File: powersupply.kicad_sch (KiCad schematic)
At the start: 94 parts, among them J201 EXT PWR, U201 TPS54332, U202 TPS54332, U203 TPS54332, U204 TPS54332

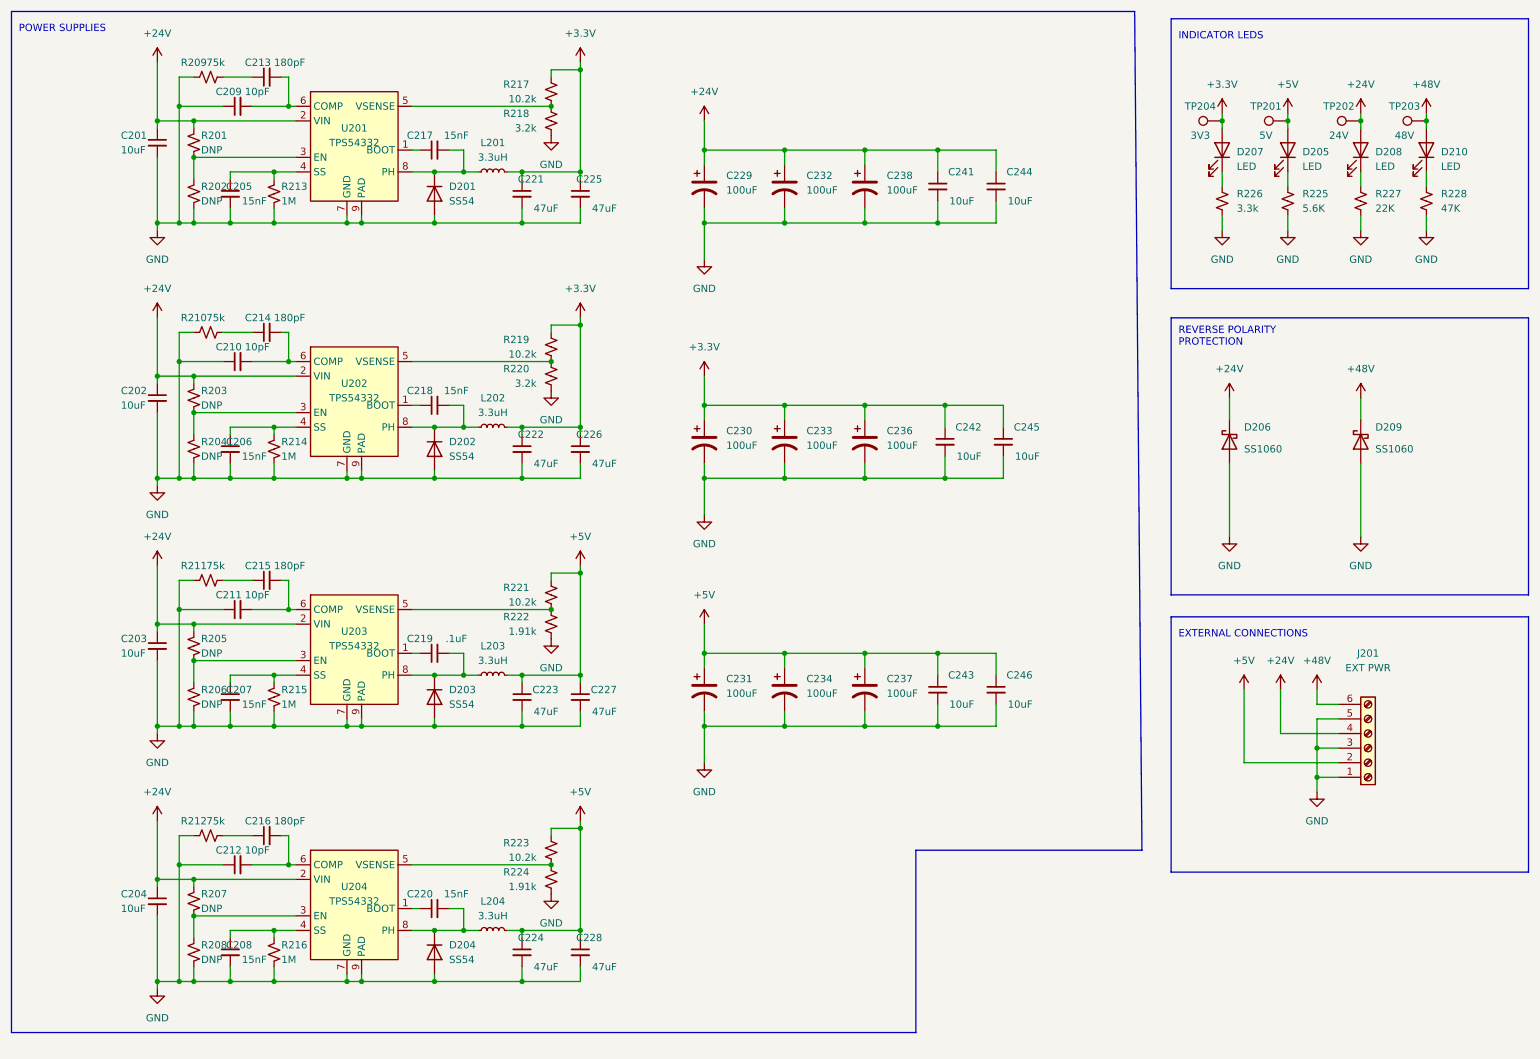
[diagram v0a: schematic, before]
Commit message: update board
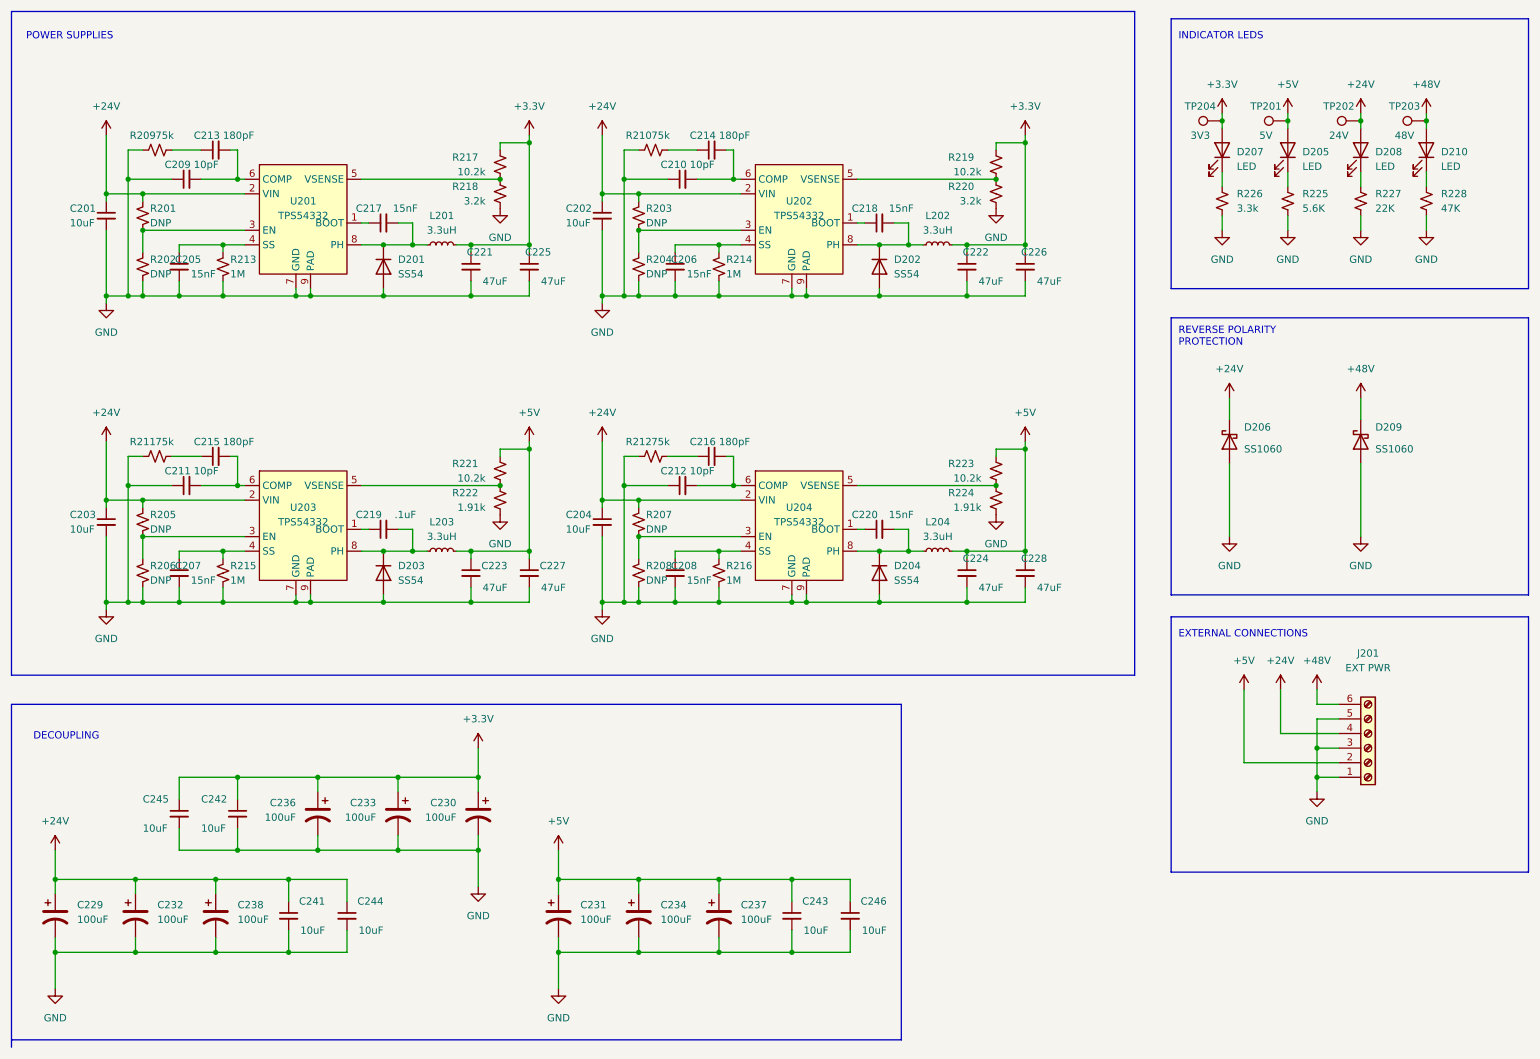
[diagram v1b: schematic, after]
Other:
- note added: "DECOUPLING"
- moved on the sheet: C201, C202, C203, C204, C205, C206, C207, C208, C209, C210, C211, C212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
